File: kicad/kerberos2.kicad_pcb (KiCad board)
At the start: 2 copper layers, 62.5 x 83.8 mm, 169 parts, among them J1 5V, J10 GND, J11 rp_spare1, J12 rp_spare2, J13 rp_spare3, J14 rp_spare4, J15 SWCLK, J16 SWD, J17 xout, J18 503398-1892, J19 MIDI-in, J2 IEC_ATN, J20 MIDI-thru, J21 MIDI-out, J3 IEC_SRQ, J4 IEC_CLK, J5 IEC_DAT, J6 GND, J7 3.3V, J8 1.2V, J9 current-measurement, SW1 side-switch, SW2 SKRPADE010, U1 MX25L25645G, U10 AD8694ARZ, U11 TMCS1108A3UQDR, U12 M3406, U13 M3406, U14 6N138, U15 74LS14, U2 MX25L25645G, U3 RP2040, U4 74LCX16245, U5 74LCX16245, U6 GW1NR-4&4B_QN881, U7 74LCX16245, U8 74LS06, U9 74LS06, X1 SX3M12.000M20F30TNN

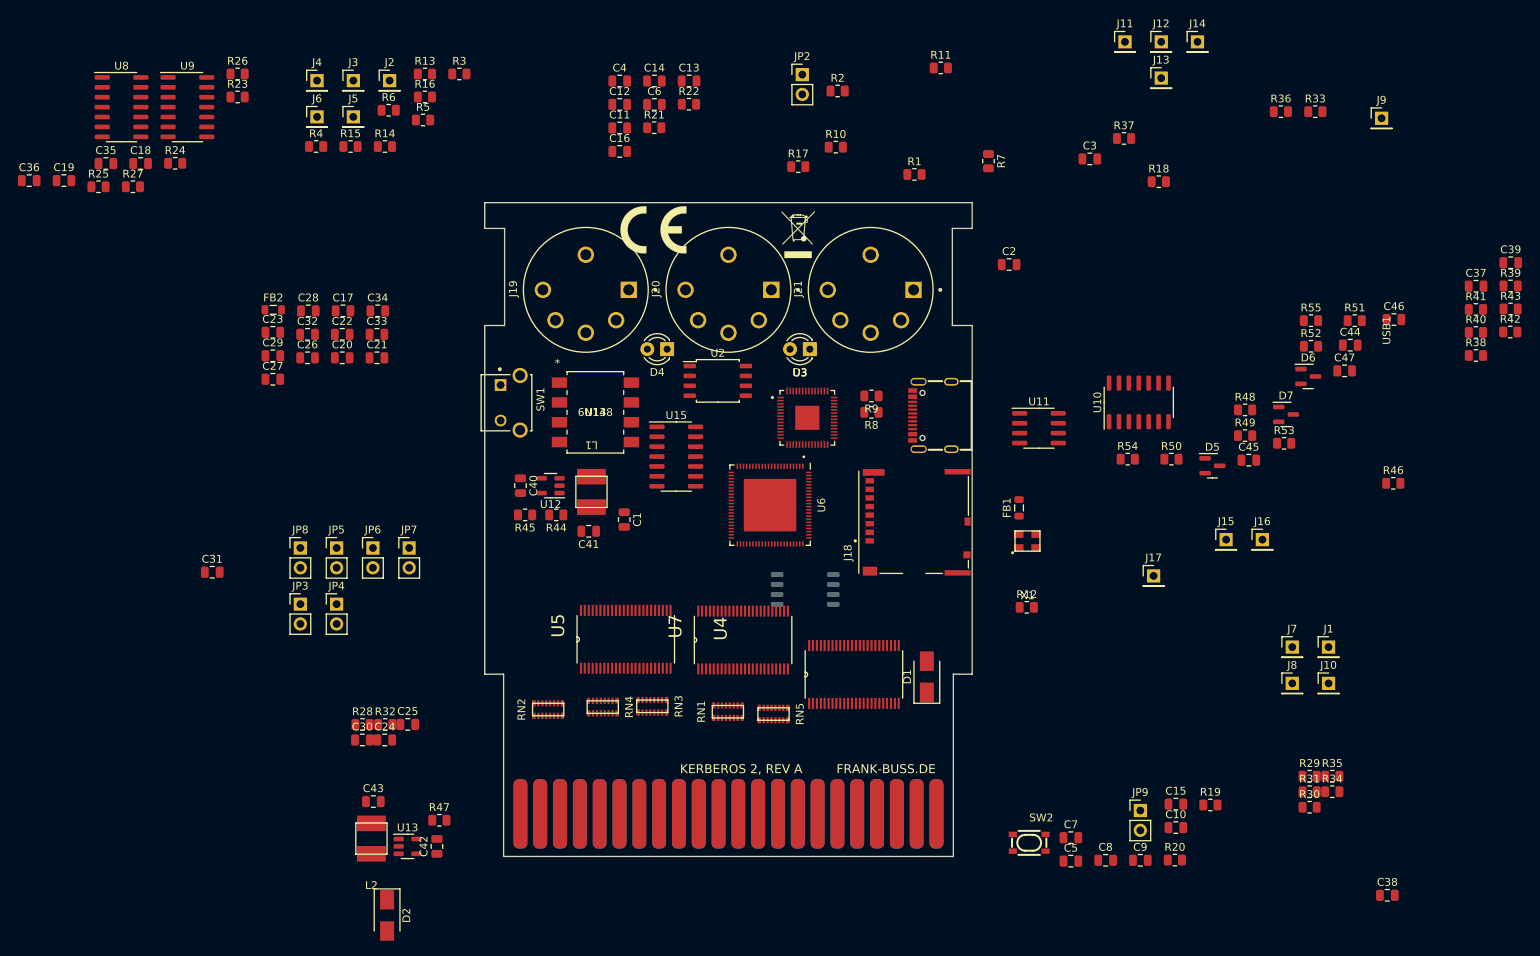
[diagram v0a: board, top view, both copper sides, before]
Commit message: started routing
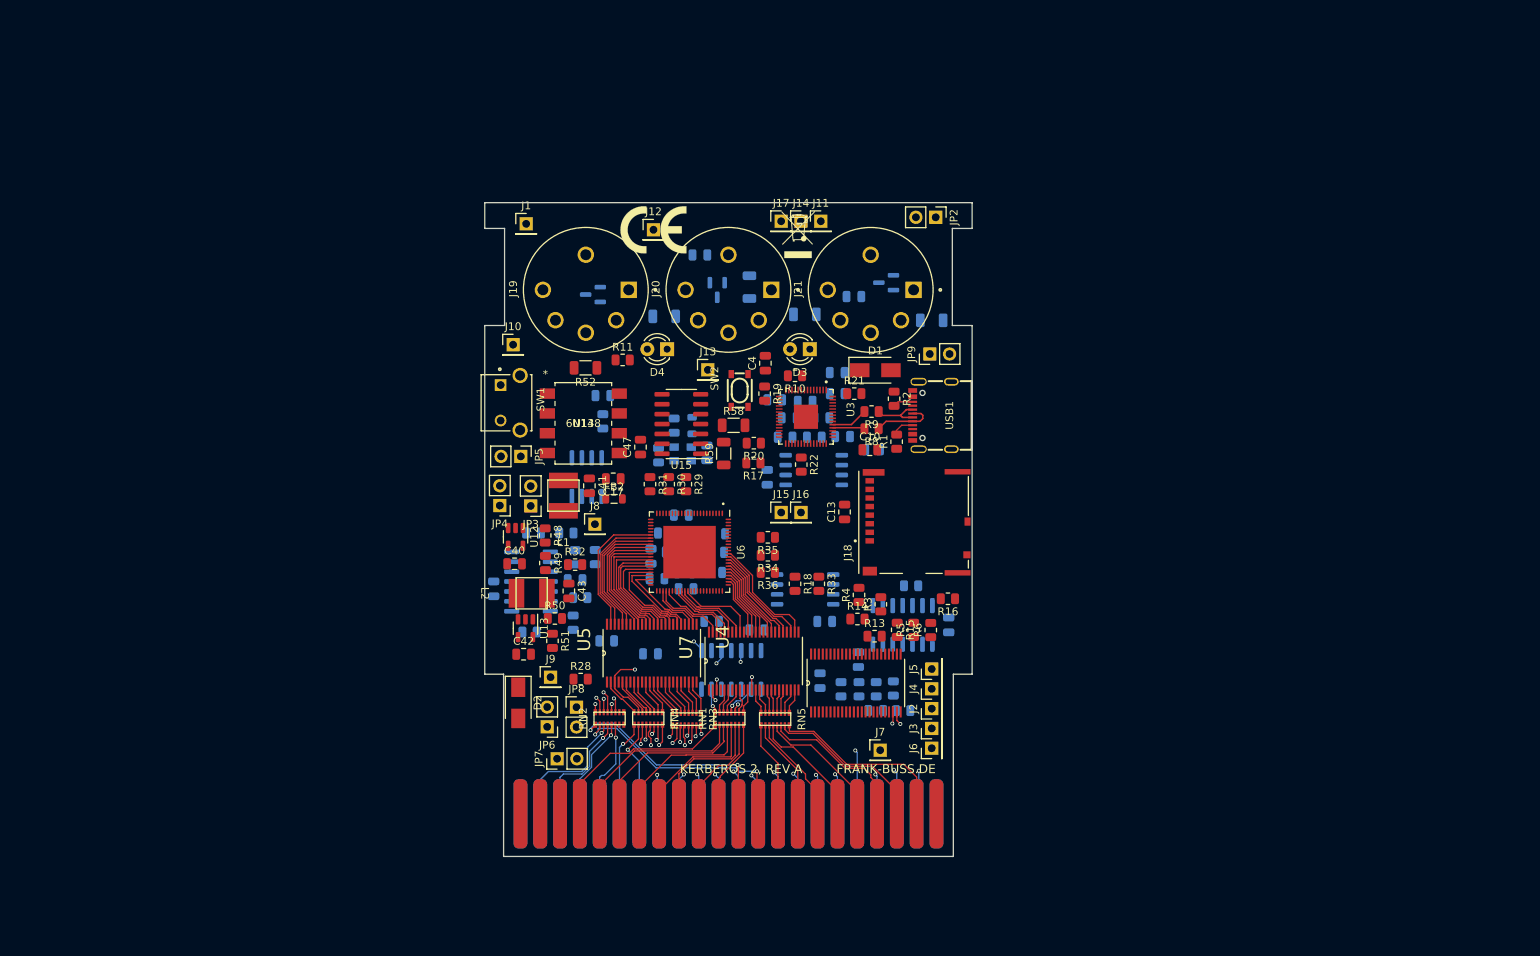
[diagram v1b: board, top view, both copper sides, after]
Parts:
- C1, C11, C12, C14, C15, C16, C18, C19, C2, C20, C21, C22, C23, C24, C25, C26, C27, C28, C29, C3, C30, C31, C32, C33, C34, C35, C36, C37, C38, C39, C44, C45, C46, C5, C6, C7, C8, C9, D5, D6, D7, FB1, R12, R23, R24, R25, R26, R27, R37, R7, U10, U11, U2, U8, U9, X1: moved to B.Cu
- R1, R2: value 5.1 -> 5k1
- R42: renamed from R38; moved to B.Cu
- R43: renamed from R39; moved to B.Cu
- R44: renamed from R40; moved to B.Cu
- R45: renamed from R41; moved to B.Cu
- R46: renamed from R42; moved to B.Cu
- R47: renamed from R43; moved to B.Cu
- R52: renamed from R48; footprint Resistor_SMD:R_0805_2012Metric -> Resistor_SMD:R_1206_3216Metric
- R53: renamed from R49; footprint Resistor_SMD:R_0805_2012Metric -> Resistor_SMD:R_1206_3216Metric; moved to B.Cu
- R54: renamed from R50; footprint Resistor_SMD:R_0805_2012Metric -> Resistor_SMD:R_1206_3216Metric; moved to B.Cu
- R55: renamed from R51; footprint Resistor_SMD:R_0805_2012Metric -> Resistor_SMD:R_1206_3216Metric; moved to B.Cu
- R56: renamed from R52; footprint Resistor_SMD:R_0805_2012Metric -> Resistor_SMD:R_1206_3216Metric; moved to B.Cu
- R57: renamed from R53; moved to B.Cu
- R58: renamed from R54; footprint Resistor_SMD:R_0805_2012Metric -> Resistor_SMD:R_1206_3216Metric
- R59: renamed from R55; footprint Resistor_SMD:R_0805_2012Metric -> Resistor_SMD:R_1206_3216Metric
- moved C39 136.9 mm to (47.0, 88.5), turned to 90 degrees
- moved R47 132.4 mm to (51.6, 94.1), turned to 180 degrees
- moved C36 130.9 mm to (105.3, 93.2), turned to -90 degrees
- moved J9 128.4 mm to (54.3, 99.8)
- moved R46 125.8 mm to (57.1, 92.9), turned to -90 degrees
- moved R43 125.1 mm to (56.3, 81.4)
- moved C37 121.5 mm to (57.4, 87.4)
- moved U8 120.2 mm to (99.4, 93.2), turned to 90 degrees
- moved R44 119.8 mm to (58.1, 89.7), turned to 180 degrees
- moved C38 118.9 mm to (52.1, 81.4), turned to 180 degrees
- moved R42 118.3 mm to (57.4, 84.5), turned to 90 degrees
- moved C18 117.5 mm to (95.9, 104.1)
- moved R45 117.3 mm to (60.0, 84.5), turned to -90 degrees
- moved R25 116.9 mm to (93.8, 101.4), turned to -90 degrees
- moved R27 116.8 mm to (98.2, 101.3), turned to -90 degrees
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- renumbered R44 to R48, R45 to R49, R46 to R50, R47 to R51
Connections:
- U3 pad 36: /GW1NR FPGA/IEC_ATN_t -> /GW1NR FPGA/IEC_DAT_t
- U3 pad 37: /GW1NR FPGA/IEC_SRQ_t -> /GW1NR FPGA/IEC_CLK_t
- U3 pad 38: /GW1NR FPGA/IEC_CLK_t -> /GW1NR FPGA/IEC_ATN_t
- U3 pad 39: /GW1NR FPGA/IEC_DAT_t -> /GW1NR FPGA/IEC_SRQ_t
- U6 pad 68: /GW1NR FPGA/D7_t -> /GW1NR FPGA/~{ROML_t}
- U6 pad 69: /GW1NR FPGA/D6_t -> /GW1NR FPGA/~{ROMH_t}
- U6 pad 70: /GW1NR FPGA/D5_t -> /GW1NR FPGA/D7_t
- U6 pad 71: /GW1NR FPGA/D4_t -> /GW1NR FPGA/D6_t
- U6 pad 72: /GW1NR FPGA/D3_t -> /GW1NR FPGA/D5_t
- U6 pad 73: /GW1NR FPGA/D2_t -> /GW1NR FPGA/D4_t
- U6 pad 74: /GW1NR FPGA/D1_t -> /GW1NR FPGA/D3_t
- U6 pad 75: /GW1NR FPGA/D0_t -> /GW1NR FPGA/D2_t
- U6 pad 76: /GW1NR FPGA/~{ROMH_t} -> /GW1NR FPGA/D1_t
- U6 pad 77: /GW1NR FPGA/~{ROML_t} -> /GW1NR FPGA/D0_t
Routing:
- net ~{RESET}: track 0.00 -> 48.4 mm, vias 0 -> 2
- net ~{NMI}: track 0.00 -> 39.6 mm, vias 0 -> 2
- net Net-(JP1-PadY): track 0.00 -> 38.5 mm, vias 0 -> 2
- net Net-(JP1-PadX): track 0.00 -> 35.8 mm, vias 0 -> 2
- net Net-(JP1-PadW): track 0.00 -> 32.9 mm, vias 0 -> 2
- net Net-(JP1-PadV): track 0.00 -> 32.0 mm, vias 0 -> 2
- net Net-(JP1-Pad13): track 0.00 -> 30.6 mm, vias 0 -> 2
- net Net-(JP1-Pad12): track 0.00 -> 28.8 mm, vias 0 -> 2
- net Net-(JP1-PadU): track 0.00 -> 28.7 mm, vias 0 -> 2
- net Net-(JP1-PadT): track 0.00 -> 26.7 mm, vias 0 -> 2
- net ~{ROMH}: track 0.00 -> 26.7 mm, vias 0 -> 2
- net Net-(JP1-PadS): track 0.00 -> 25.0 mm, vias 0 -> 2
- net Net-(JP1-Pad4): track 0.00 -> 24.4 mm
- net Net-(JP1-Pad21): track 0.00 -> 24.2 mm
- net Net-(JP1-Pad5): track 0.00 -> 23.6 mm
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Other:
- copper layers 2 -> 4
